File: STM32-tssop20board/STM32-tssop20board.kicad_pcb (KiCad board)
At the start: 2 copper layers, 19.2 x 53.9 mm, 25 parts, among them J1 Conn_01x10_Male, J2 Conn_01x10_Male, J3 Conn_01x03_Male, J4 USB_A, J5 USB_B_Micro, J6 Target_SWD, J7 IF_SWD, J8 Target_UART, SW1 Reset, U1 STM32F042F6Px, U2 MCP1700-3302E_SOT23, Y1 8M

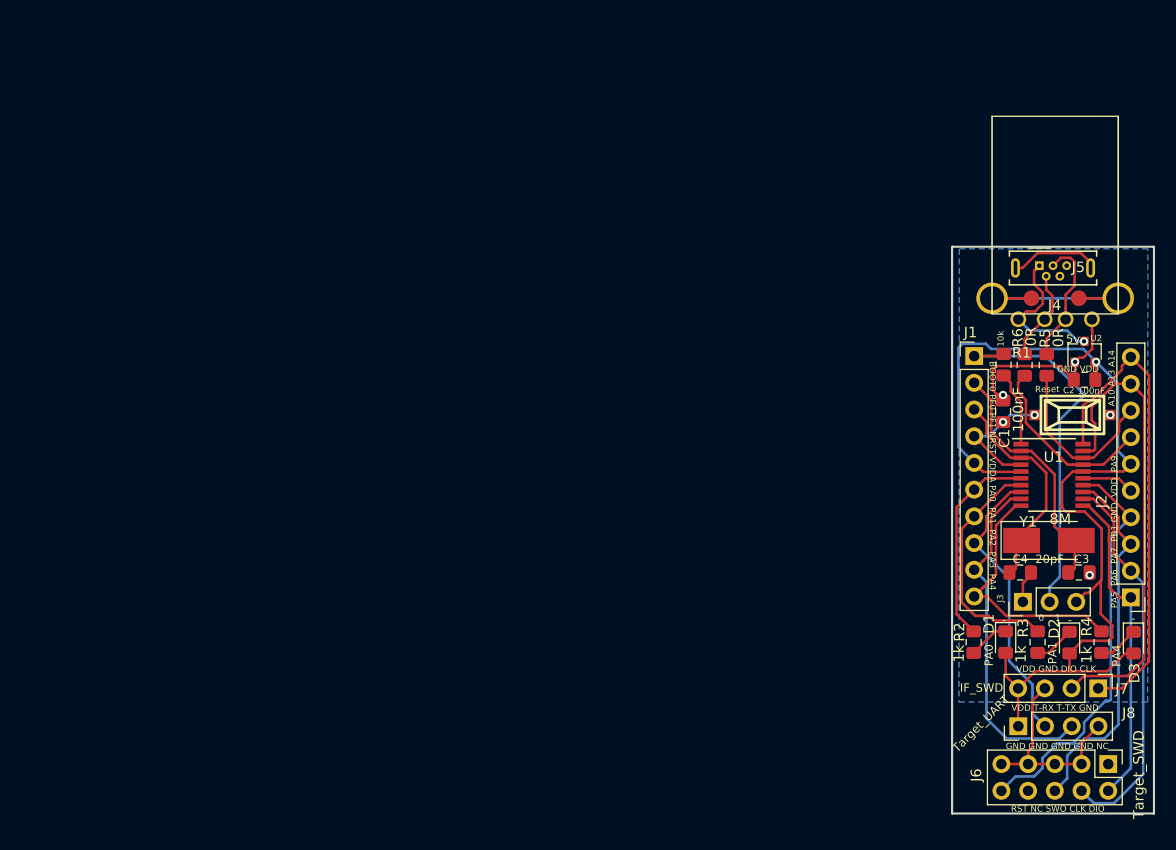
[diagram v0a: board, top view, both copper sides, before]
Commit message: Update for some staged changes. Not sure what has changed actually
Signed-off-by: Zamir SUN <sztsian@gmail.com>
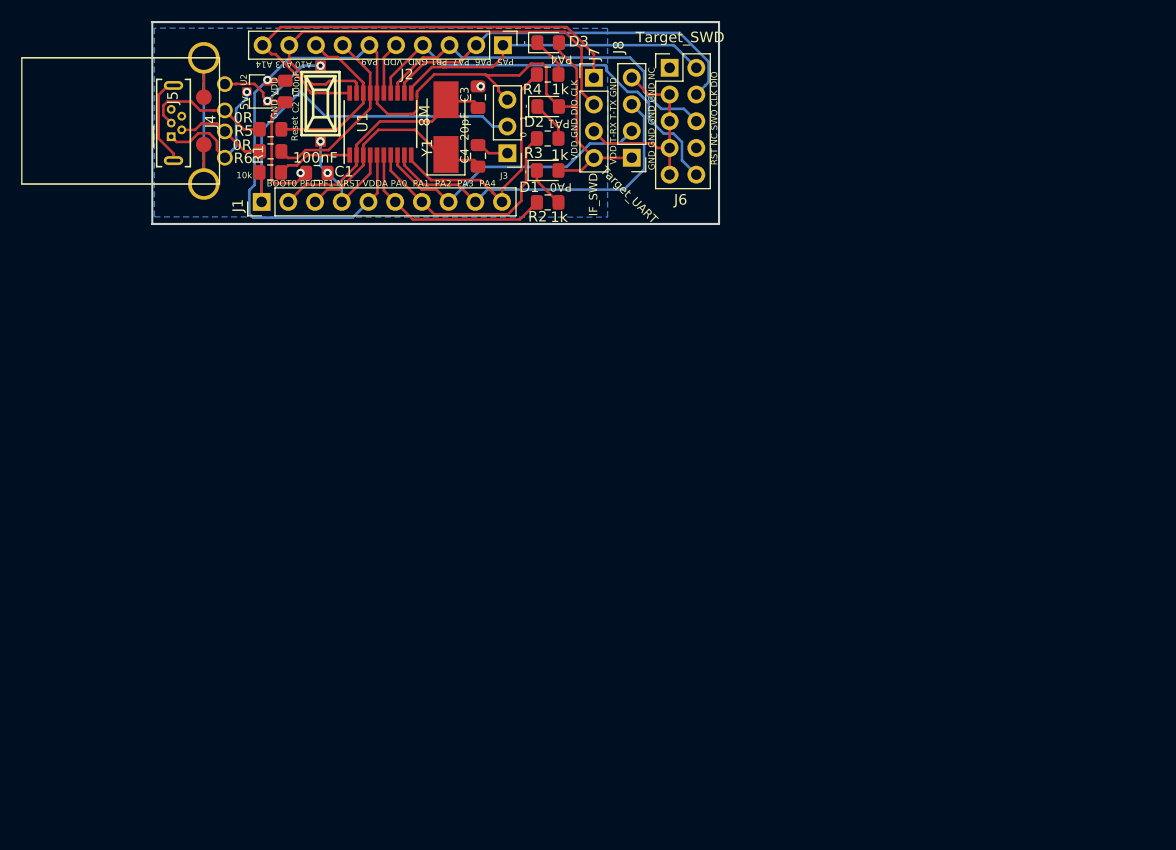
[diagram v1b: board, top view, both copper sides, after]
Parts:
- moved J4 85.4 mm to (65.8, 34.8), turned to 270 degrees
- moved J5 83.5 mm to (60.7, 39.8), turned to 90 degrees
- moved U2 82.5 mm to (68.9, 35.5), turned to 180 degrees
- moved C2 80.8 mm to (71.6, 35.5), turned to 270 degrees
- moved D3 79.7 mm to (96.6, 30.9), turned to 0 degrees
- moved J2 79.5 mm to (92.3, 31.1), turned to 270 degrees
- moved J6 78.3 mm to (108.1, 33.3), turned to 0 degrees
- moved SW1 77.4 mm to (74.9, 36.7), turned to 270 degrees
- moved R5 77.1 mm to (70.2, 39.1), turned to 180 degrees
- moved R4 75.4 mm to (96.5, 33.9), turned to 0 degrees
- moved J7 75.3 mm to (100.9, 34.2), turned to 0 degrees
- moved R6 74.5 mm to (70.2, 41.2), turned to 180 degrees
- moved C3 72.9 mm to (89.9, 36.1), turned to 90 degrees
- moved R1 72.1 mm to (70.2, 43.2), turned to 0 degrees
- moved U1 72.1 mm to (80.6, 38.6), turned to 90 degrees
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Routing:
- net GND: track 45.9 -> 52.3 mm
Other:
- board size 19.2 x 53.9 mm -> 53.9 x 19.2 mm
